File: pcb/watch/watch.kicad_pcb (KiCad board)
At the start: 8 copper layers, 28 x 34.4 mm, 98 parts, among them U1 STM32G031K8Ux, U2 TLV74130PDQNR

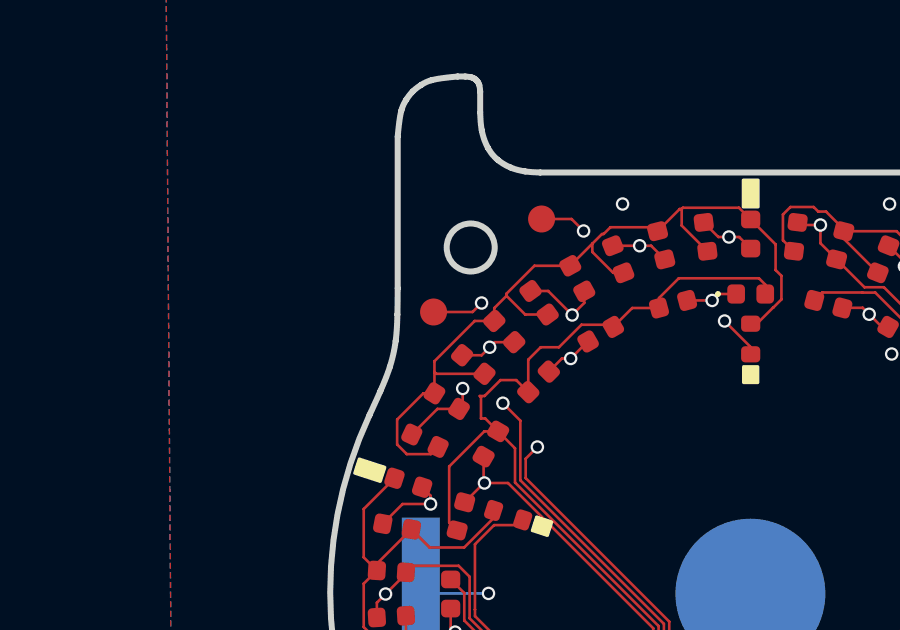
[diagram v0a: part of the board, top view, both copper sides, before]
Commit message: e
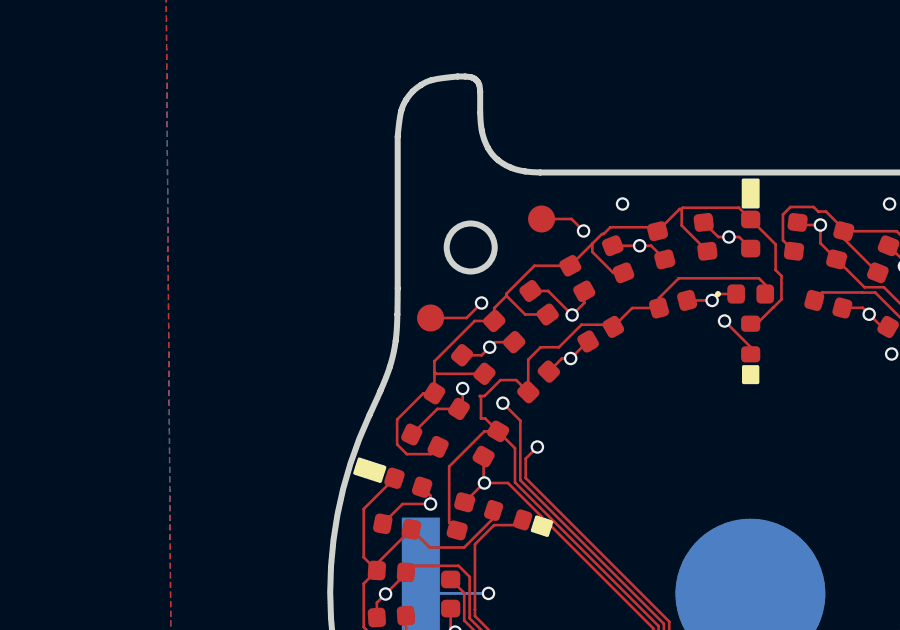
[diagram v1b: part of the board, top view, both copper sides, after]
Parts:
- moved TP6 0.22 mm to (39.3, 27.3)
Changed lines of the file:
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@@
   )
   (footprint "footprints:testpoint_better" (layer "F.Cu")
-    (at 39.4 27.1)
+    (at 39.3 27.3)
     (descr "SMD pad as test Point, diameter 1.0mm")
     (tags "test point SMD pad")
@@
   (segment (start 50.98665 44.20665) (end 50.72 43.94) (width 0.0889) (layer "F.Cu") (net 34))
   (segment (start 47.0778 38.7953) (end 47.0778 37.494904) (width 0.0889) (layer "F.Cu") (net 36))
-  (segment (start 41 26.8) (end 40.7 27.1) (width 0.0889) (layer "F.Cu") (net 36))
   (segment (start 47.0778 37.494904) (end 42.2922 32.709304) (width 0.0889) (layer "F.Cu") (net 36))
+  (segment (start 39.3 27.3) (end 40.5 27.3) (width 0.0889) (layer "F.Cu") (net 36))
+  (segment (start 40.5 27.3) (end 41 26.8) (width 0.0889) (layer "F.Cu") (net 36))
   (segment (start 47.5325 39.25) (end 47.0778 38.7953) (width 0.0889) (layer "F.Cu") (net 36))
   (segment (start 42.2922 32.709304) (end 42.2922 30.7222) (width 0.0889) (layer "F.Cu") (net 36))
   (segment (start 42.2922 30.7222) (end 41.71 30.14) (width 0.0889) (layer "F.Cu") (net 36))
-  (segment (start 40.7 27.1) (end 39.4 27.1) (width 0.0889) (layer "F.Cu") (net 36))
   (via (at 41.71 30.14) (size 0.45) (drill 0.3) (layers "F.Cu" "B.Cu") (net 36))
   (via (at 41 26.8) (size 0.45) (drill 0.3) (layers "F.Cu" "B.Cu") (net 36))
